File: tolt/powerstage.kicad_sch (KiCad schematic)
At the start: 146 parts, among them Q1 NMOS, Q10 NMOS, Q11 NMOS, Q12 NMOS, Q13 NMOS, Q14 NMOS, Q15 NMOS, Q16 NMOS, Q17 NMOS, Q18 NMOS, Q2 NMOS, Q3 NMOS, Q4 NMOS, Q5 NMOS, Q6 NMOS, Q7 NMOS, Q8 NMOS, Q9 NMOS

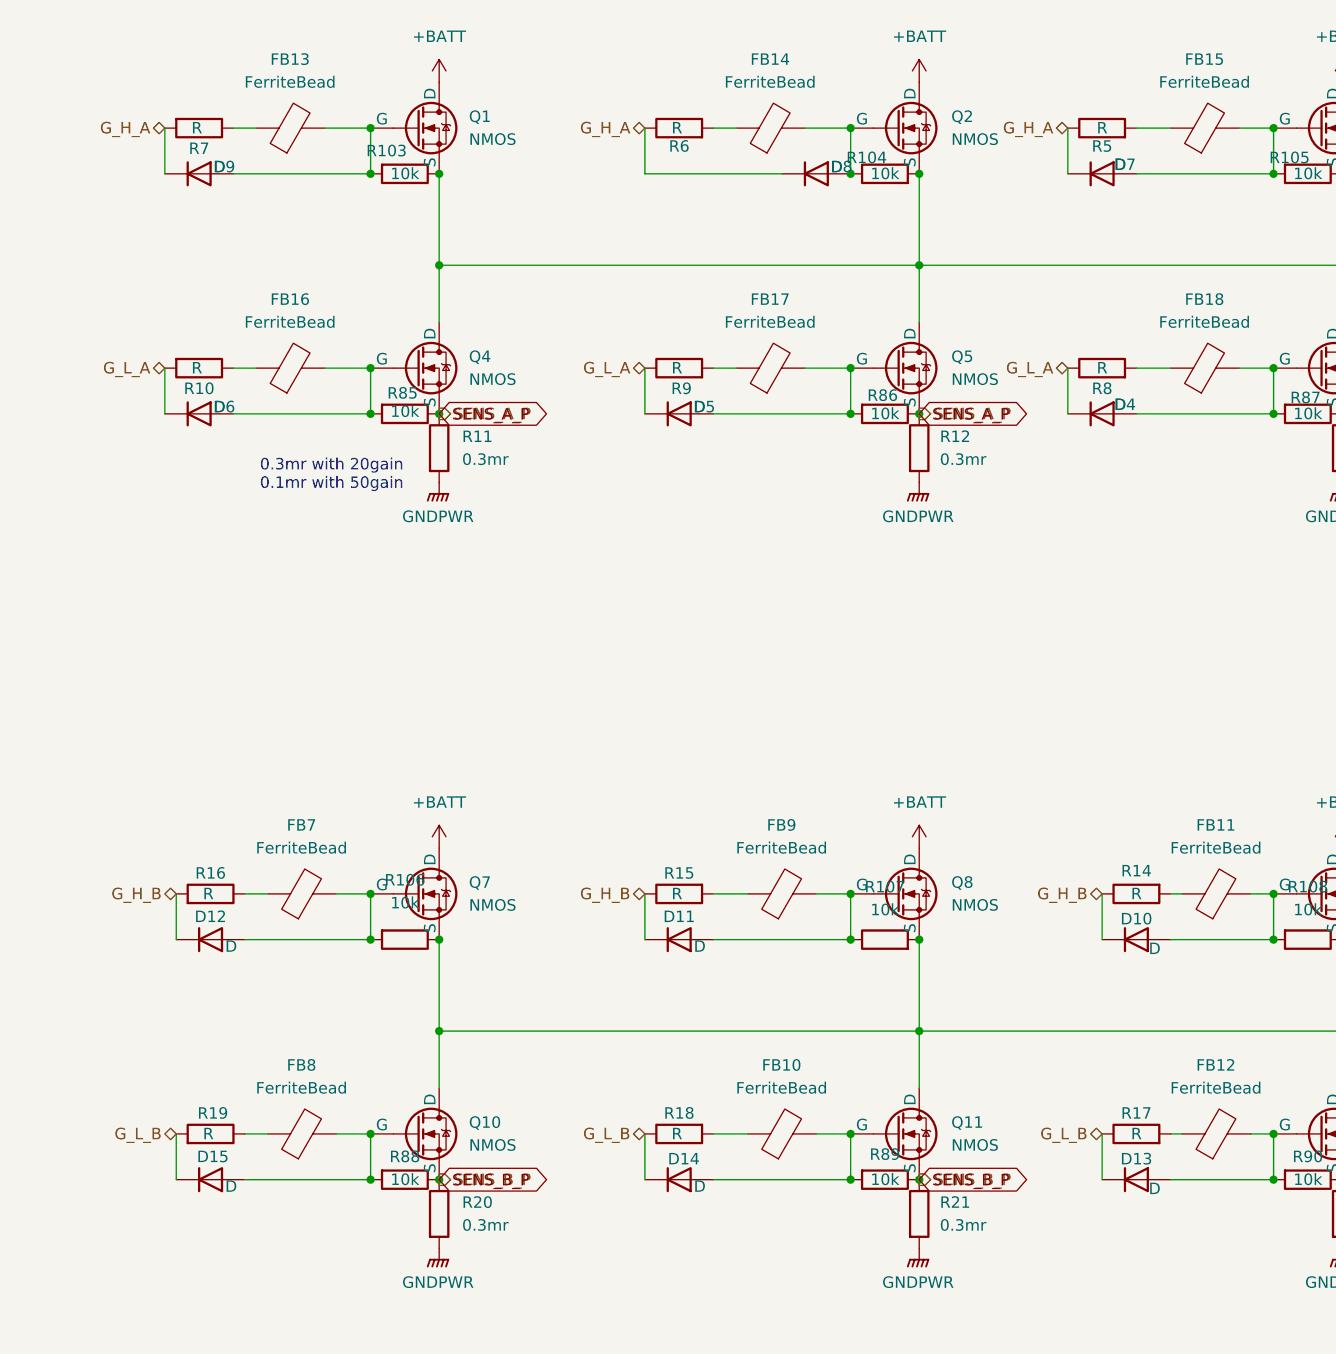
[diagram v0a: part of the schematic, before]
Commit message: begenning of lcsc part assign
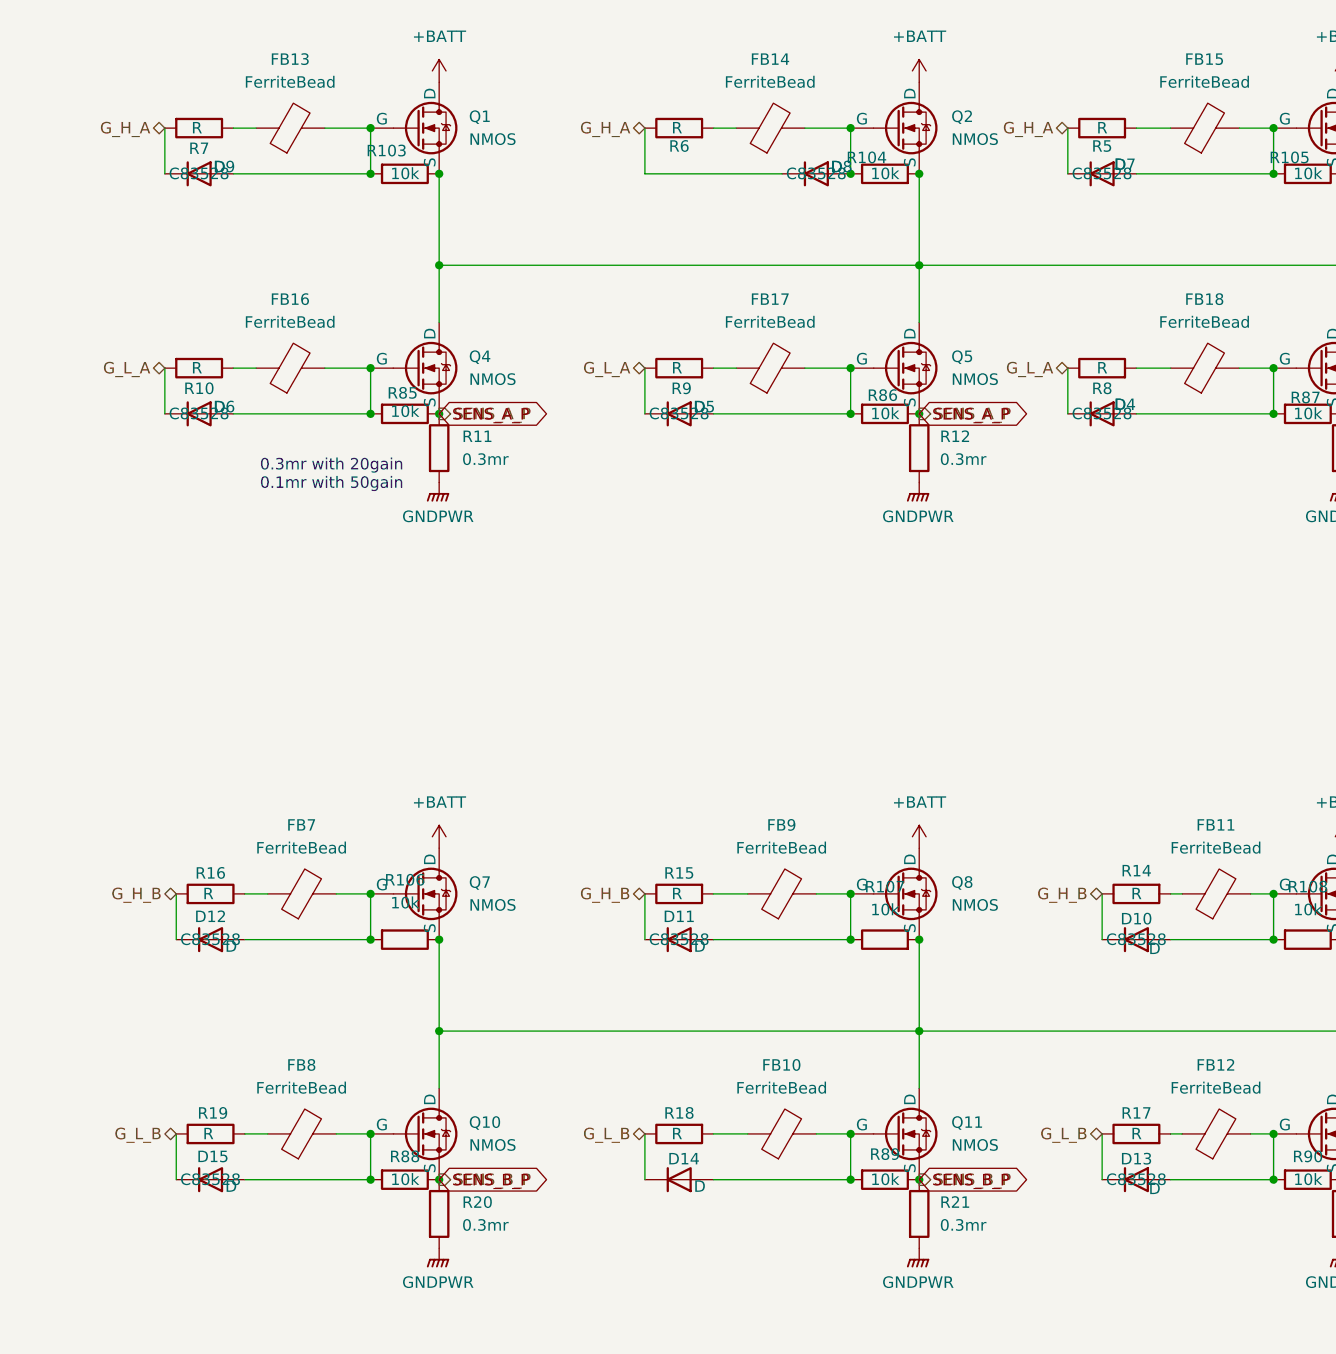
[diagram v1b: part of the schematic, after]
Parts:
- C101, C103, C104, C106, C107, C108, C109, C110, C112, C113, C114, C115, C128, C129, C130, C131, C132, C133, C134, C135, C136, C137, C138, C139, C140, C141, C142: footprint Capacitor_SMD:C_2220_5750Metric_Pad1.97x5.40mm_HandSolder -> Capacitor_SMD:C_2220_5750Metric
- D10, D11, D12, D13, D14, D15, D16, D17, D18, D19, D20, D21, D4, D5, D6, D7, D8, D9: LCSC (none) -> C83528
- FB1, FB10, FB11, FB12, FB13, FB14, FB15, FB16, FB17, FB18, FB2, FB3, FB4, FB5, FB6, FB7, FB8, FB9: footprint (none) -> Capacitor_SMD:C_0603_1608Metric
- R103, R104, R105, R106, R107, R108, R109, R110, R111, R61, R62, R63, R85, R86, R87, R88, R89, R90, R91, R92, R93: LCSC (none) -> C25804
